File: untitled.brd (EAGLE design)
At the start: 100 x 50 mm, 20 parts, among them Q1 IRF740, Q2 IRF740

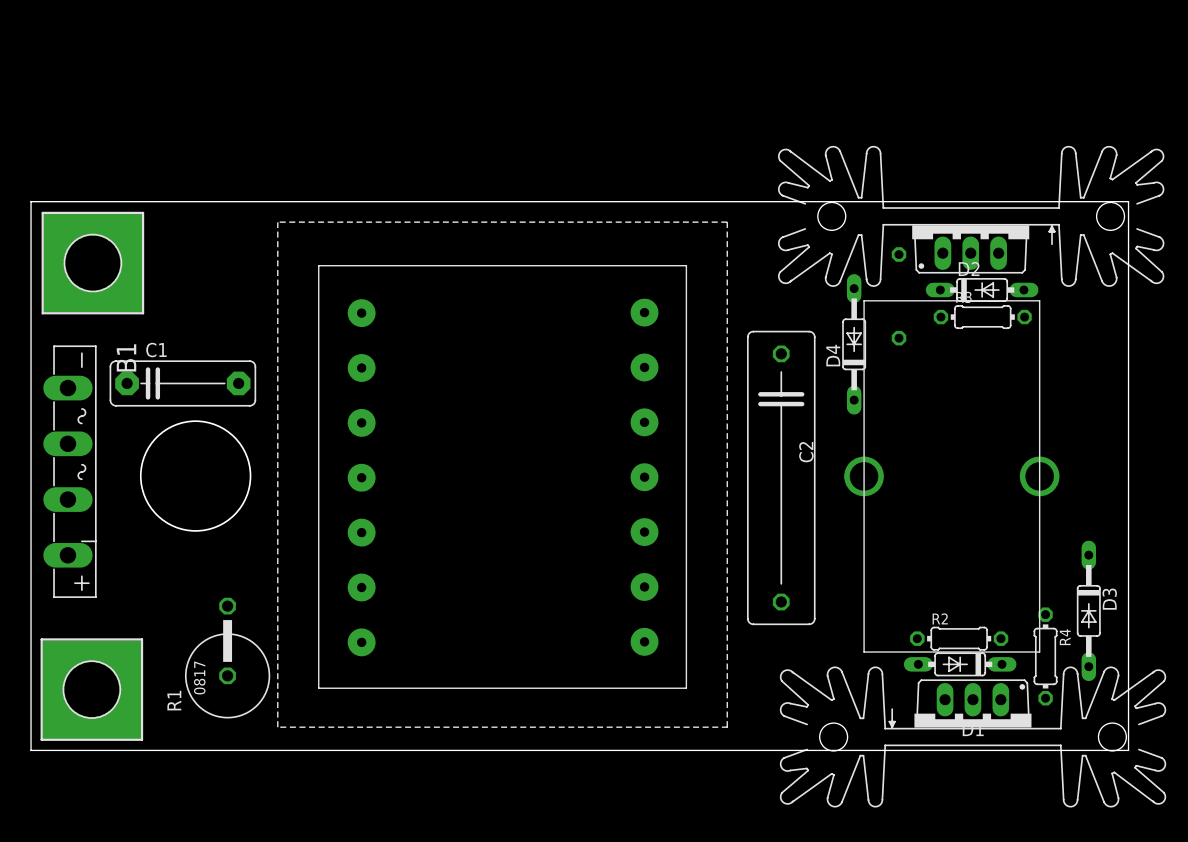
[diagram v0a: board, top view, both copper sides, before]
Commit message: add
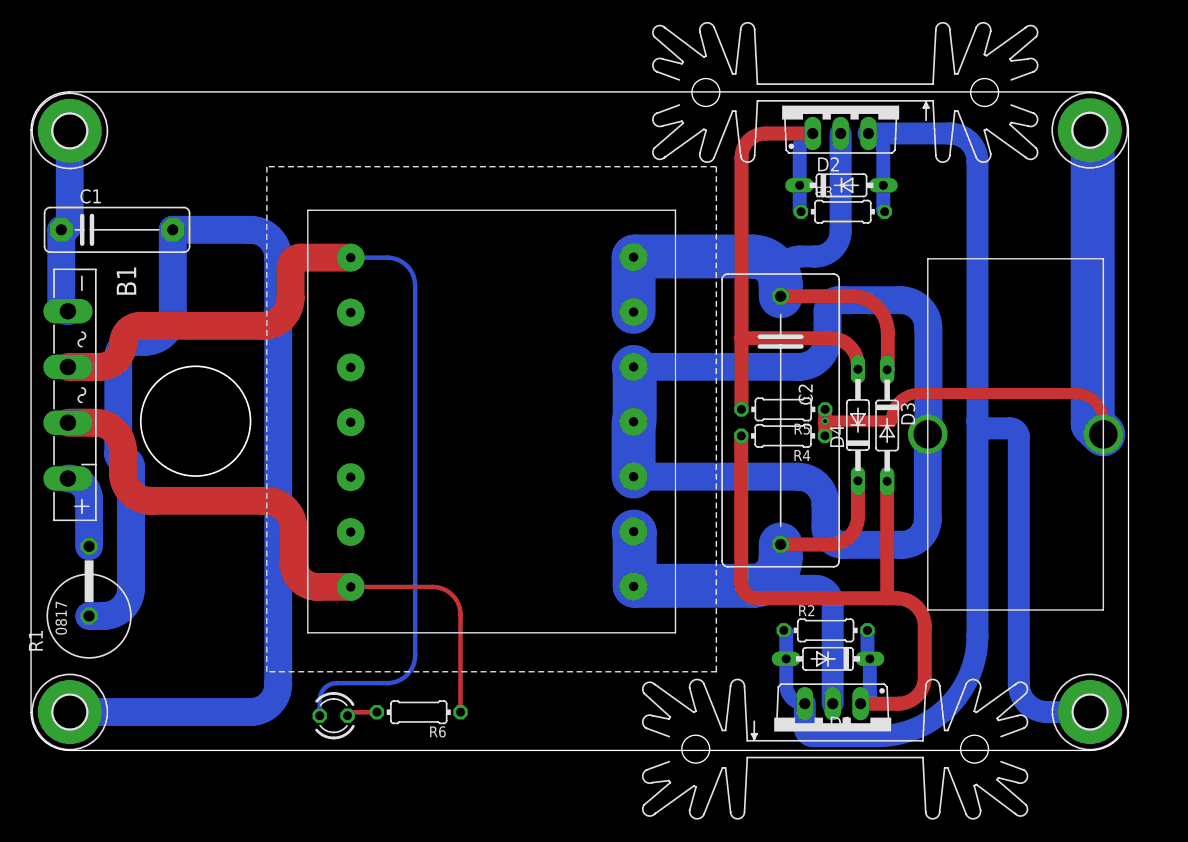
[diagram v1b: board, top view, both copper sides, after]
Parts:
- added GND2, VCC-BT: MOUNT-PAD-ROUND3.0, holes:3,0-PAD
- added LED1: TLLR4400, led:LED3MM
- added R6: 1m, rcl:0204/7
- C2: device rcl:C225-062X268 -> rcl:C225-108X268
- GND, VCC: value MOUNT-PAD-SQUARE5.0 -> MOUNT-PAD-ROUND3.0; device holes:5,0-PAD-SQUARE -> holes:3,0-PAD
- moved R4 31.2 mm to (68.5, 28.7), turned to 180 degrees
- moved D3 25.0 mm to (78.0, 29.6)
- moved Q2 16.1 mm to (73.8, 58.8)
- moved U$2 16.1 mm to (74.2, 59.2)
- moved D2 16.0 mm to (73.8, 51.5)
- moved R3 16.0 mm to (74.0, 49.1)
- moved C1 15.2 mm to (7.84, 47.4)
- moved R5 14.7 mm to (68.5, 31.1), flipped to the top, turned to 180 degrees
- moved R1 13.7 mm to (5.29, 17.3)
- moved Q1 12.8 mm to (73.0, 1.72)
- moved U$3 12.6 mm to (73.3, 0.88)
- moved GND 12.2 mm to (3.53, 56.4)
- moved R2 12.2 mm to (72.4, 10.9)
- moved D1 12.0 mm to (72.6, 8.34)
- moved D4 7.36 mm to (75.3, 29.6)
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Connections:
- removed net VCC: R4.1, R5.1, U$4.P$2
- new net N$8: R4.1, R5.1, U$4.P$2, VCC-BT.B3,0
- new net N$9: LED1.A, R6.2
- net GND: now also GND2.B3,0, R3.2
- net N$1: now also LED1.K
- net N$2: now also R6.1
- net N$3: now also GND.B3,0; no longer GND.B5
- net N$4: now also VCC.B3,0; no longer VCC.B5
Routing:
- net GND: track 0.00 -> 126.2 mm
- net N$4: track 0.00 -> 110.3 mm
- net T4-2: track 0.00 -> 90.9 mm
- net N$1: track 0.00 -> 83.9 mm
- net N$6: track 0.00 -> 61.0 mm
- net N$8: track 0.00 -> 59.7 mm, vias 0 -> 1
- net N$2: track 0.00 -> 54.9 mm
- net O2: track 0.00 -> 53.0 mm
- net N$7: track 0.00 -> 50.0 mm
- net O1: track 0.00 -> 49.0 mm
- net N$3: track 0.00 -> 17.0 mm
- net N$5: track 0.00 -> 6.98 mm
- net N$9: track 0.00 -> 2.80 mm
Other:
- board size 100 x 50 mm -> 100 x 60 mm
